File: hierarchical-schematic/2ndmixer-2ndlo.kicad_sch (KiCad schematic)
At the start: 58 parts

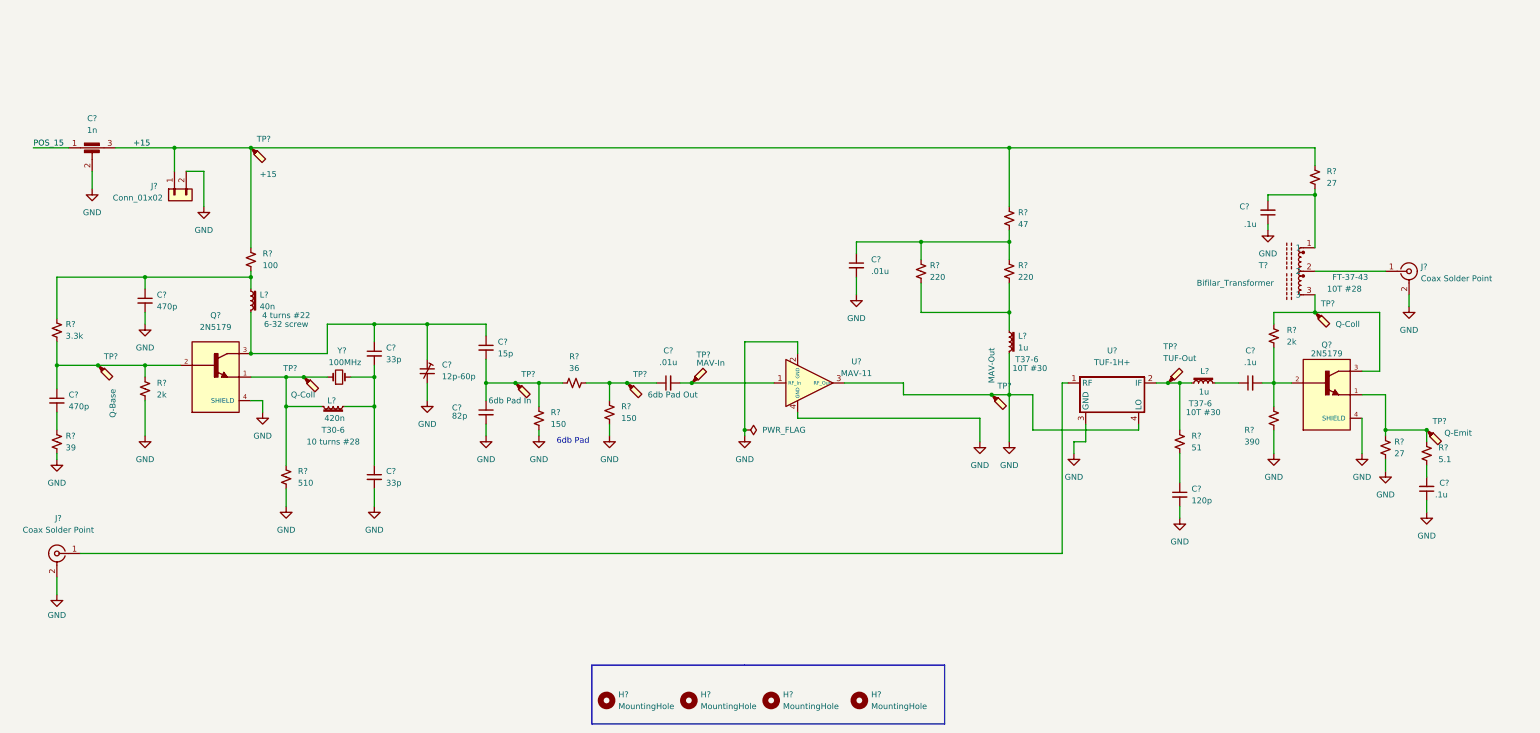
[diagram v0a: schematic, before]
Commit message: v7 conversion
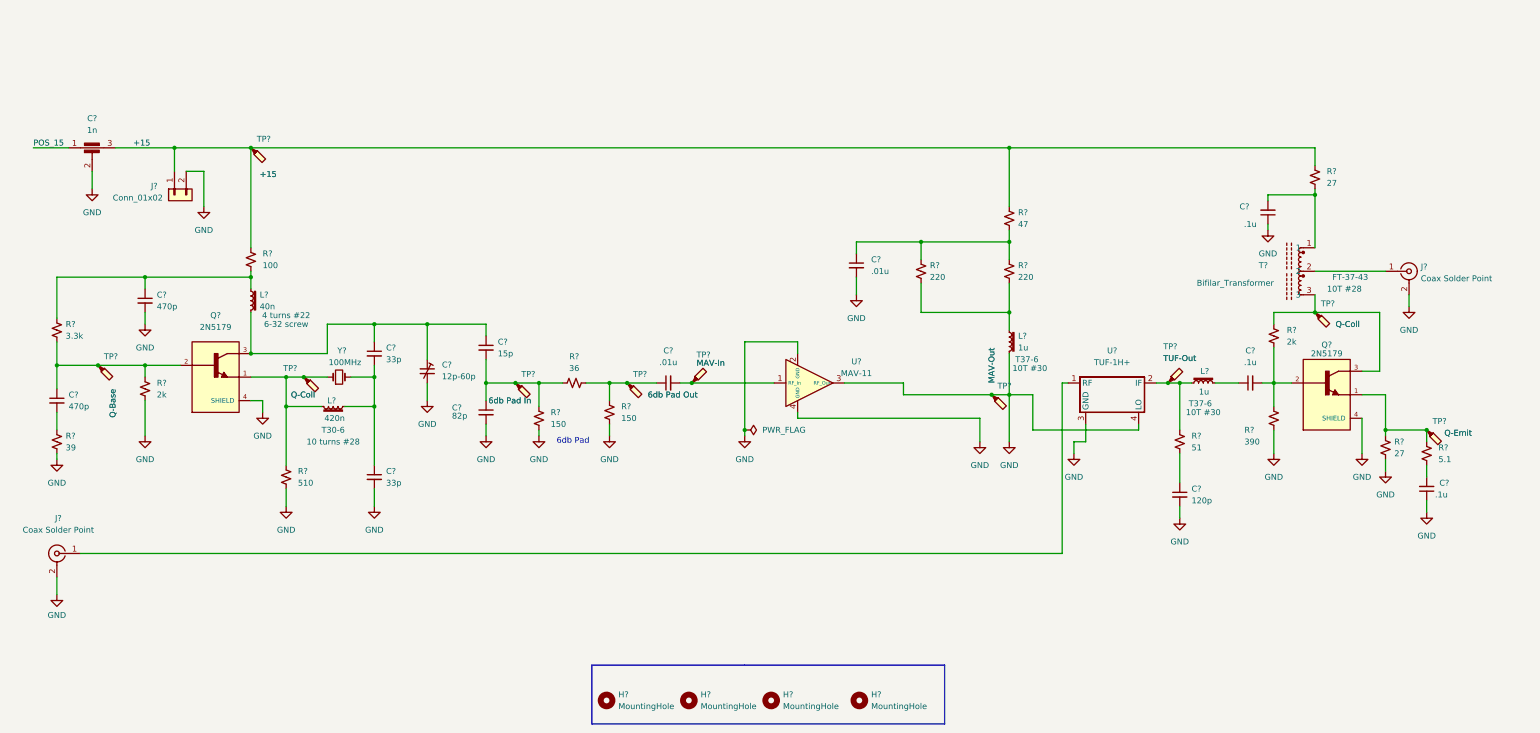
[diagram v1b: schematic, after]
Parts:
- J? (x2): Spice_Model Conn_Coaxial -> (none); Spice_Netlist_Enabled N -> (none); Spice_Primitive J -> (none)
- J?: Spice_Model Conn_01x02 -> (none); Spice_Netlist_Enabled N -> (none); Spice_Primitive J -> (none)
- Q? (x2): Spice_Lib_File 2ndmixer-2ndlo-spice\2N5179.LIB -> (none); Spice_Model 2N5179 -> (none); Spice_Netlist_Enabled Y -> (none); Spice_Primitive Q -> (none)
- TP? (x2): value Q-Coll -> ${SIM.PARAMS}; Spice_Netlist_Enabled N -> (none)
- TP?: value 6db Pad Out -> ${SIM.PARAMS}; Spice_Netlist_Enabled N -> (none)
- TP?: value MAV-Out -> ${SIM.PARAMS}; Spice_Netlist_Enabled N -> (none)
- TP?: value Q-Emit -> ${SIM.PARAMS}; Spice_Netlist_Enabled N -> (none)
- TP?: value +15 -> ${SIM.PARAMS}; Spice_Netlist_Enabled N -> (none)
- TP?: value 6db Pad In -> ${SIM.PARAMS}; Spice_Netlist_Enabled N -> (none)
- TP?: value Q-Base -> ${SIM.PARAMS}; Spice_Netlist_Enabled N -> (none)
- TP?: value TUF-Out -> ${SIM.PARAMS}; Spice_Netlist_Enabled N -> (none)
- TP?: value MAV-In -> ${SIM.PARAMS}; Spice_Netlist_Enabled N -> (none)

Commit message: 2ndmixer-2ndlo rev 1
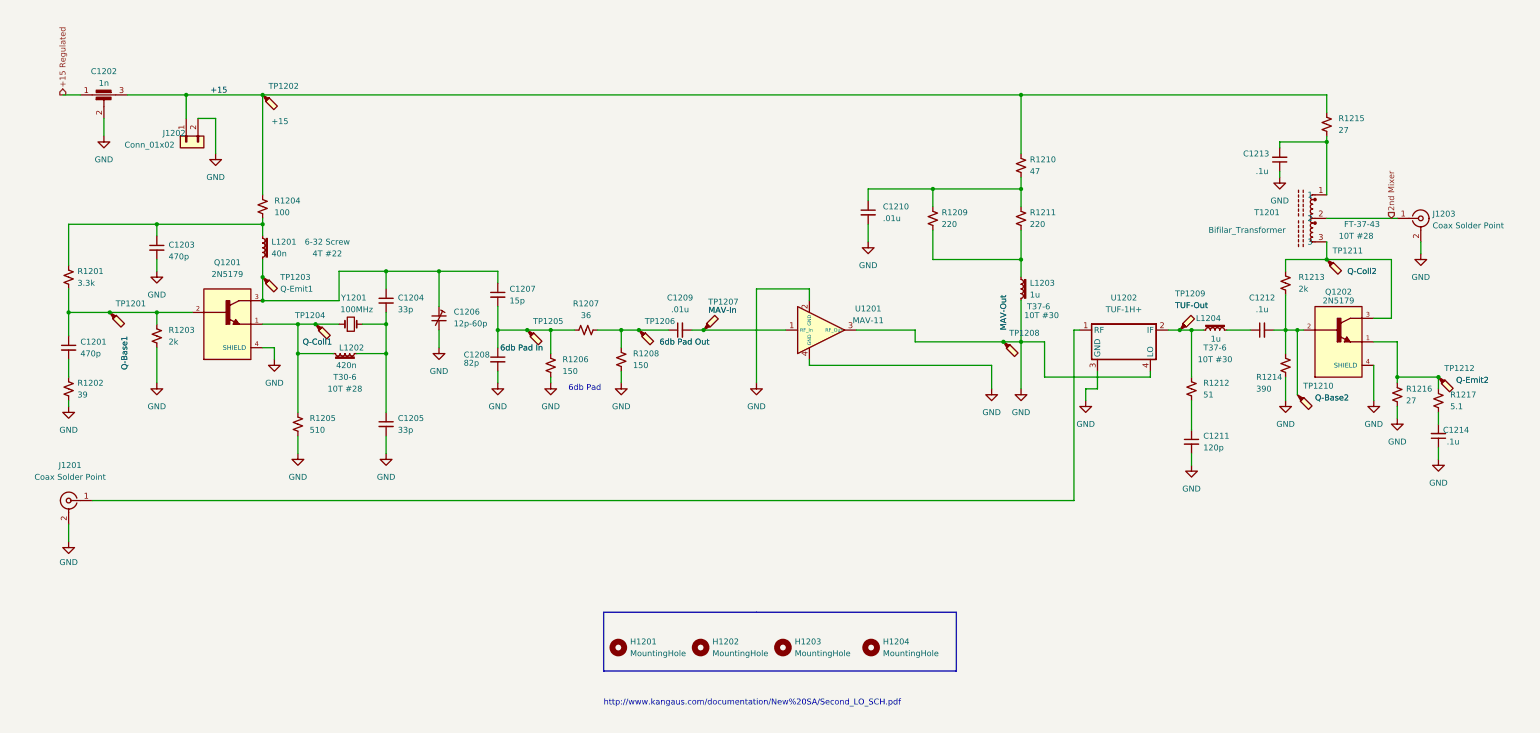
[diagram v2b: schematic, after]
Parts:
- removed C? (x3): .1u, Capacitor_THT:C_Disc_D5.0mm_W2.5mm_P5.00mm, symbol Device:C_Small
- removed C?: 15p, Capacitor_THT:C_Disc_D5.0mm_W2.5mm_P5.00mm, symbol Device:C_Small
- removed C?: 120p, Capacitor_THT:C_Disc_D5.0mm_W2.5mm_P5.00mm, symbol Device:C_Small
- removed C? (x2): 33p, Capacitor_THT:C_Disc_D5.0mm_W2.5mm_P5.00mm, symbol Device:C_Small
- removed C?: 1n, 2ndmixer-2ndlo:DSS1NB32A102Q91A, symbol Device:C_Feedthrough
- removed C?: 82p, Capacitor_THT:C_Disc_D5.0mm_W2.5mm_P5.00mm, symbol Device:C_Small
- removed C?: 12p-60p, 2ndmixer-2ndlo:GKG60015, symbol Device:C_Trim_Small
- removed C? (x2): 470p, Capacitor_THT:C_Disc_D5.0mm_W2.5mm_P5.00mm, symbol Device:C_Small
- removed C? (x2): .01u, Capacitor_THT:C_Disc_D5.0mm_W2.5mm_P5.00mm, symbol Device:C_Small
- removed H? (x4): MountingHole, MountingHole:MountingHole_3.2mm_M3, symbol Mechanical:MountingHole
- removed J? (x2): Coax Solder Point, Connector_Wire:SolderWire-0.5sqmm_1x02_P4.6mm_D0.9mm_OD2.1mm, symbol Connector:Conn_Coaxial
- removed J?: Conn_01x02, 2ndmixer-2ndlo:691103110002, symbol Connector_Generic:Conn_01x02
- removed L?: 40n, Inductor_THT:L_Toroid_Vertical_L13.0mm_W6.5mm_P5.60mm, symbol Device:L_Iron_Small
- removed L?: 420n, Inductor_THT:L_Toroid_Vertical_L13.0mm_W6.5mm_P5.60mm, symbol Device:L_Iron_Small
- removed L? (x2): 1u, Inductor_THT:L_Toroid_Vertical_L13.0mm_W6.5mm_P5.60mm, symbol Device:L_Iron_Small
- removed Q?: 2N5179, TO127P584H533-4N, symbol spectrum_analyzer:2N5179
- removed Q?: 2N5179, 2ndmixer-2ndlo:TO127P584H533-4N, symbol 2ndmixer-2ndlo:2N5179
- removed R?: 100, Resistor_THT:R_Axial_DIN0207_L6.3mm_D2.5mm_P7.62mm_Horizontal, symbol Device:R_Small_US
- removed R?: 47, Resistor_THT:R_Axial_DIN0207_L6.3mm_D2.5mm_P7.62mm_Horizontal, symbol Device:R_Small_US
- removed R? (x2): 220, Resistor_THT:R_Axial_DIN0207_L6.3mm_D2.5mm_P7.62mm_Horizontal, symbol Device:R_Small_US
- removed R? (x2): 27, Resistor_THT:R_Axial_DIN0207_L6.3mm_D2.5mm_P7.62mm_Horizontal, symbol Device:R_Small_US
- removed R? (x2): 150, Resistor_THT:R_Axial_DIN0207_L6.3mm_D2.5mm_P7.62mm_Horizontal, symbol Device:R_Small_US
- removed R? (x2): 2k, Resistor_THT:R_Axial_DIN0207_L6.3mm_D2.5mm_P7.62mm_Horizontal, symbol Device:R_Small_US
- removed R?: 51, Resistor_THT:R_Axial_DIN0207_L6.3mm_D2.5mm_P7.62mm_Horizontal, symbol Device:R_Small_US
- removed R?: 390, Resistor_THT:R_Axial_DIN0207_L6.3mm_D2.5mm_P7.62mm_Horizontal, symbol Device:R_Small_US
- removed R?: 3.3k, Resistor_THT:R_Axial_DIN0207_L6.3mm_D2.5mm_P7.62mm_Horizontal, symbol Device:R_Small_US
- removed R?: 36, Resistor_THT:R_Axial_DIN0207_L6.3mm_D2.5mm_P7.62mm_Horizontal, symbol Device:R_Small_US
- removed R?: 510, Resistor_THT:R_Axial_DIN0207_L6.3mm_D2.5mm_P7.62mm_Horizontal, symbol Device:R_Small_US
- removed R?: 39, Resistor_THT:R_Axial_DIN0207_L6.3mm_D2.5mm_P7.62mm_Horizontal, symbol Device:R_Small_US
- removed R?: 5.1, Resistor_THT:R_Axial_DIN0207_L6.3mm_D2.5mm_P7.62mm_Horizontal, symbol Device:R_Small_US
- removed T?: Bifilar_Transformer, Transformer_THT:Autotransformer_Toroid_1Tap_Horizontal_D10.5mm_Amidon-T37, symbol spectrum_analyzer:Bifilar_Transformer
- removed TP? (x10): ${SIM.PARAMS}, TestPoint:TestPoint_Pad_1.0x1.0mm, symbol Connector:TestPoint_Probe
- removed U?: MAV-11, 2ndmixer-2ndlo:MAV-11BSM&plus_, symbol spectrum_analyzer:MAV-11
- removed U?: TUF-1H+, 2ndmixer-2ndlo:TUF-1H, symbol spectrum_analyzer:TUF-1H+
- removed Y?: 100MHz, Crystal:Crystal_HC49-U_Vertical, symbol Device:Crystal_Small
- added C1201, C1203: 470p, Capacitor_THT:C_Disc_D5.0mm_W2.5mm_P5.00mm, symbol Device:C_Small
- added C1202: 1n, spectrum_analyzer:DSS1NB32A102Q91A, symbol Device:C_Feedthrough
- added C1204, C1205: 33p, Capacitor_THT:C_Disc_D5.0mm_W2.5mm_P5.00mm, symbol Device:C_Small
- added C1206: 12p-60p, spectrum_analyzer:GKG60015, symbol Device:C_Trim_Small
- added C1207: 15p, Capacitor_THT:C_Disc_D5.0mm_W2.5mm_P5.00mm, symbol Device:C_Small
- added C1208: 82p, Capacitor_THT:C_Disc_D5.0mm_W2.5mm_P5.00mm, symbol Device:C_Small
- added C1209, C1210: .01u, Capacitor_THT:C_Disc_D5.0mm_W2.5mm_P5.00mm, symbol Device:C_Small
- added C1211: 120p, Capacitor_THT:C_Disc_D5.0mm_W2.5mm_P5.00mm, symbol Device:C_Small
- added C1212, C1213, C1214: .1u, Capacitor_THT:C_Disc_D5.0mm_W2.5mm_P5.00mm, symbol Device:C_Small
- added H1201, H1202, H1203, H1204: MountingHole, MountingHole:MountingHole_3.2mm_M3, symbol Mechanical:MountingHole
- added J1201, J1203: Coax Solder Point, Connector_Wire:SolderWire-0.5sqmm_1x02_P4.6mm_D0.9mm_OD2.1mm, symbol Connector:Conn_Coaxial
- added J1202: Conn_01x02, spectrum_analyzer:691103110002, symbol Connector_Generic:Conn_01x02
- added L1201: 40n, Inductor_THT:L_Toroid_Vertical_L13.0mm_W6.5mm_P5.60mm, symbol Device:L_Iron_Small
- added L1202: 420n, Inductor_THT:L_Toroid_Vertical_L13.0mm_W6.5mm_P5.60mm, symbol Device:L_Iron_Small
- added L1203, L1204: 1u, Inductor_THT:L_Toroid_Vertical_L13.0mm_W6.5mm_P5.60mm, symbol Device:L_Iron_Small
- added Q1201: 2N5179, spectrum_analyzer:TO127P584H533-4N, symbol spectrum_analyzer:2N5179
- added Q1202: 2N5179, TO127P584H533-4N, symbol spectrum_analyzer:2N5179
- added R1201: 3.3k, Resistor_THT:R_Axial_DIN0207_L6.3mm_D2.5mm_P7.62mm_Horizontal, symbol Device:R_Small_US
- added R1202: 39, Resistor_THT:R_Axial_DIN0207_L6.3mm_D2.5mm_P7.62mm_Horizontal, symbol Device:R_Small_US
- added R1203, R1213: 2k, Resistor_THT:R_Axial_DIN0207_L6.3mm_D2.5mm_P7.62mm_Horizontal, symbol Device:R_Small_US
- added R1204: 100, Resistor_THT:R_Axial_DIN0207_L6.3mm_D2.5mm_P7.62mm_Horizontal, symbol Device:R_Small_US
- added R1205: 510, Resistor_THT:R_Axial_DIN0207_L6.3mm_D2.5mm_P7.62mm_Horizontal, symbol Device:R_Small_US
- added R1206, R1208: 150, Resistor_THT:R_Axial_DIN0207_L6.3mm_D2.5mm_P7.62mm_Horizontal, symbol Device:R_Small_US
- added R1207: 36, Resistor_THT:R_Axial_DIN0207_L6.3mm_D2.5mm_P7.62mm_Horizontal, symbol Device:R_Small_US
- added R1209, R1211: 220, Resistor_THT:R_Axial_DIN0207_L6.3mm_D2.5mm_P7.62mm_Horizontal, symbol Device:R_Small_US
- added R1210: 47, Resistor_THT:R_Axial_DIN0207_L6.3mm_D2.5mm_P7.62mm_Horizontal, symbol Device:R_Small_US
- added R1212: 51, Resistor_THT:R_Axial_DIN0207_L6.3mm_D2.5mm_P7.62mm_Horizontal, symbol Device:R_Small_US
- added R1214: 390, Resistor_THT:R_Axial_DIN0207_L6.3mm_D2.5mm_P7.62mm_Horizontal, symbol Device:R_Small_US
- added R1215, R1216: 27, Resistor_THT:R_Axial_DIN0207_L6.3mm_D2.5mm_P7.62mm_Horizontal, symbol Device:R_Small_US
- added R1217: 5.1, Resistor_THT:R_Axial_DIN0207_L6.3mm_D2.5mm_P7.62mm_Horizontal, symbol Device:R_Small_US
- added T1201: Bifilar_Transformer, Transformer_THT:Autotransformer_Toroid_1Tap_Horizontal_D10.5mm_Amidon-T37, symbol spectrum_analyzer:Bifilar_Transformer
- added TP1201: Q-Base1, TestPoint:TestPoint_Pad_1.0x1.0mm, symbol Connector:TestPoint_Probe
- added TP1202: +15, TestPoint:TestPoint_Pad_1.0x1.0mm, symbol Connector:TestPoint_Probe
- added TP1203: Q-Emit1, TestPoint:TestPoint_Pad_1.0x1.0mm, symbol Connector:TestPoint_Probe
- added TP1204: Q-Coll1, TestPoint:TestPoint_Pad_1.0x1.0mm, symbol Connector:TestPoint_Probe
- added TP1205: 6db Pad In, TestPoint:TestPoint_Pad_1.0x1.0mm, symbol Connector:TestPoint_Probe
- added TP1206: 6db Pad Out, TestPoint:TestPoint_Pad_1.0x1.0mm, symbol Connector:TestPoint_Probe
- added TP1207: MAV-In, TestPoint:TestPoint_Pad_1.0x1.0mm, symbol Connector:TestPoint_Probe
- added TP1208: MAV-Out, TestPoint:TestPoint_Pad_1.0x1.0mm, symbol Connector:TestPoint_Probe
- added TP1209: TUF-Out, TestPoint:TestPoint_Pad_1.0x1.0mm, symbol Connector:TestPoint_Probe
- added TP1210: Q-Base2, TestPoint:TestPoint_Pad_1.0x1.0mm, symbol Connector:TestPoint_Probe
- added TP1211: Q-Coll2, TestPoint:TestPoint_Pad_1.0x1.0mm, symbol Connector:TestPoint_Probe
- added TP1212: Q-Emit2, TestPoint:TestPoint_Pad_1.0x1.0mm, symbol Connector:TestPoint_Probe
- added U1201: MAV-11, spectrum_analyzer:MAV-11BSM&plus_, symbol spectrum_analyzer:MAV-11
- added U1202: TUF-1H+, spectrum_analyzer:TUF-1H, symbol spectrum_analyzer:TUF-1H+
- added Y1201: 100MHz, Crystal:Crystal_HC49-U_Vertical, symbol Device:Crystal_Small
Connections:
- net +15: now also C1202.3, J1202.1 (Pin_1), R1204.1, R1210.1, R1215.1, TP1202.1
- net GND: now also C1202.2, C1203.2, C1205.2, C1206.2, C1208.2, C1210.2, C1211.2, C1213.1, C1214.1, J1201.2 (Ext), J1202.2 (Pin_2), J1203.2 (Ext), L1203.2, Q1201.4 (SHIELD), Q1202.4 (SHIELD), R1202.2, R1203.2, R1205.2, R1206.2, R1208.2, R1214.2, R1216.2, TP1208.1, U1201.2 (GND), U1201.3 (RF_Out), U1201.4 (GND), U1202.3 (GND), U1202.4 (LO)
- new net: J1201.1 (In), U1202.1 (RF)
- new net: L1204.1, R1212.1, TP1209.1, U1202.2 (IF)
- new net: C1210.1, R1209.1, R1210.2, R1211.1
- new net: C1209.2, TP1207.1, U1201.1 (RF_In)
- new net: C1204.2, C1205.1, L1202.1, Y1201.2
- new net: L1202.2, Q1201.1, R1205.1, TP1204.1, Y1201.1
- new net: Q1202.3, R1213.1, T1201.3, TP1211.1
- new net: C1212.2, Q1202.2, R1213.2, R1214.1, TP1210.1
- new net: C1209.1, R1207.2, R1208.1, TP1206.1
- new net: C1214.2, R1217.2
- new net: L1203.1, R1209.2, R1211.2
- new net: C1212.1, L1204.2
- new net: C1203.1, L1201.1, R1201.1, R1204.2
- new net: C1201.1, Q1201.2, R1201.2, R1203.1, TP1201.1
- new net: C1204.1, C1206.1, C1207.1, L1201.2, Q1201.3, TP1203.1
- new net: C1207.2, C1208.1, R1206.1, R1207.1, TP1205.1
- new net: C1201.2, R1202.1
- new net: C1213.2, R1215.2, T1201.1
- new net: C1211.1, R1212.2
- new net: Q1202.1, R1216.1, R1217.1, TP1212.1
- new net +15 Regulated: C1202.1
- new net 2nd Mixer: J1203.1 (In), T1201.2
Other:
- note added: "http://www.kangaus.com/documentation/New%20SA/Second_LO_SCH.pdf"
